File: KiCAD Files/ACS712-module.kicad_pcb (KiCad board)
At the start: 2 copper layers, 70 x 55 mm, 25 parts, among them J1 Banana plug, J2 Banana plug, J5 Barrel_Jack_MountingPin, U1 ACS712, U2 AMS1117-5.0

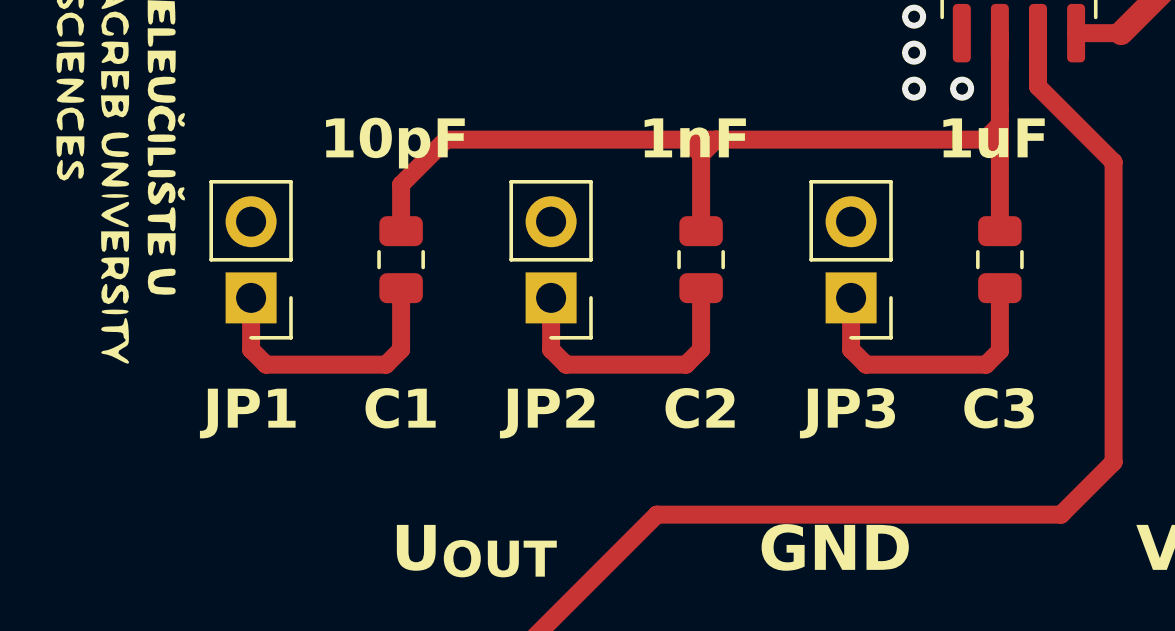
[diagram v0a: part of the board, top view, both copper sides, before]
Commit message: update
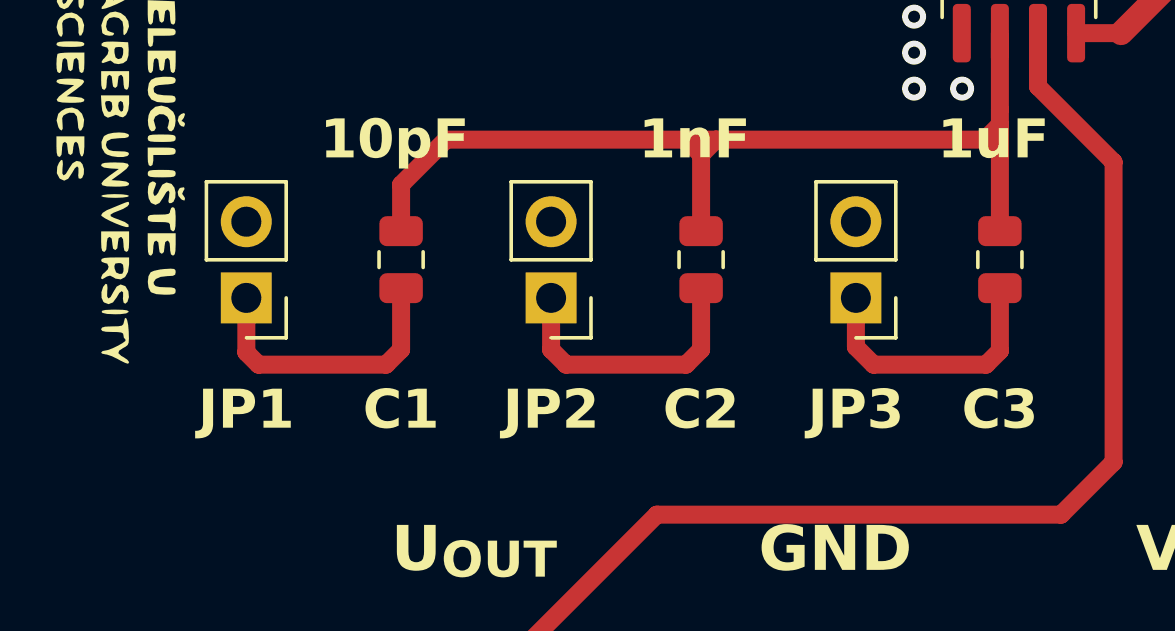
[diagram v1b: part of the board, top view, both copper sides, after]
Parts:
- moved JP1 0.16 mm to (119.3, 105.8)
- moved JP3 0.16 mm to (139.7, 105.8)
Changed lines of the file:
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@@
 	(footprint "Connector_PinHeader_2.54mm:PinHeader_1x02_P2.54mm_Vertical"
 		(layer "F.Cu")
-		(at 119.5 105.775 180)
+		(at 119.34 105.775 180)
 		(descr "Through hole straight pin header, 1x02, 2.54mm pitch, single row")
 		(tags "Through hole pin header THT 1x02 2.54mm single row")
@@
 	(footprint "Connector_PinHeader_2.54mm:PinHeader_1x02_P2.54mm_Vertical"
 		(layer "F.Cu")
-		(at 139.5 105.775 180)
+		(at 139.66 105.775 180)
 		(descr "Through hole straight pin header, 1x02, 2.54mm pitch, single row")
 		(tags "Through hole pin header THT 1x02 2.54mm single row")
@@
 	)
 	(segment
-		(start 124.5 105.45)
-		(end 124.5 107.5)
+		(start 119.75 108)
+		(end 119.34 107.59)
 		(width 0.6)
 		(layer "F.Cu")
@@
 	)
 	(segment
-		(start 124 108)
+		(start 124.5 105.45)
 		(end 124.5 107.5)
 		(width 0.6)
@@
 	)
 	(segment
-		(start 119.5 105.775)
-		(end 119.5 107.5)
+		(start 124 108)
+		(end 124.5 107.5)
 		(width 0.6)
 		(layer "F.Cu")
@@
 	)
 	(segment
-		(start 120 108)
-		(end 124 108)
+		(start 124 108)
+		(end 119.75 108)
 		(width 0.6)
 		(layer "F.Cu")
@@
 	)
 	(segment
-		(start 119.5 107.5)
-		(end 120 108)
+		(start 119.34 107.59)
+		(end 119.34 105.775)
 		(width 0.6)
 		(layer "F.Cu")
@@
 	)
 	(segment
-		(start 139.5 105.775)
-		(end 139.5 107.5)
+		(start 144 108)
+		(end 140.25 108)
 		(width 0.6)
 		(layer "F.Cu")
@@
 	)
 	(segment
-		(start 139.5 107.5)
-		(end 140 108)
+		(start 144 108)
+		(end 144.46 107.54)
 		(width 0.6)
 		(layer "F.Cu")
@@
 	)
 	(segment
-		(start 144 108)
-		(end 144.46 107.54)
+		(start 139.66 107.41)
+		(end 139.66 105.775)
 		(width 0.6)
 		(layer "F.Cu")
@@
 	)
 	(segment
-		(start 140 108)
-		(end 144 108)
+		(start 140.25 108)
+		(end 139.66 107.41)
 		(width 0.6)
 		(layer "F.Cu")
